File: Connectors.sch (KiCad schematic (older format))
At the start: 4 parts

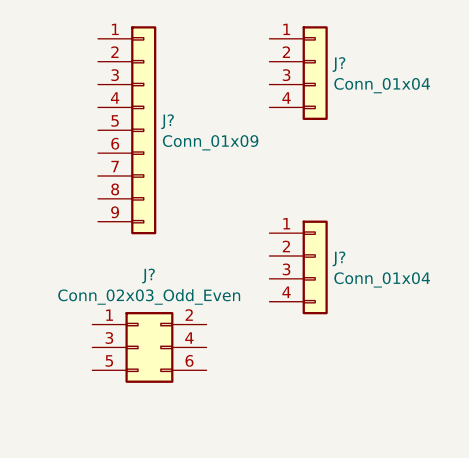
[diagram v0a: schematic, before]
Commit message: Arranged symbols
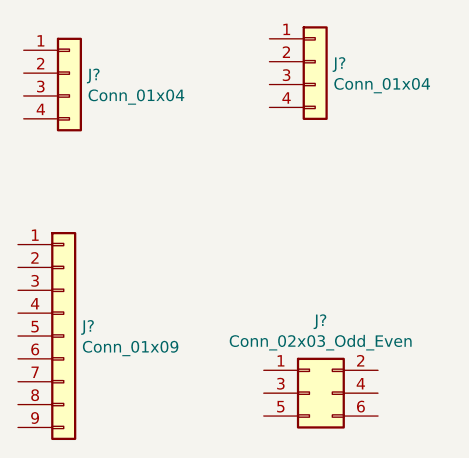
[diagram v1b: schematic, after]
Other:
- moved on the sheet: J?
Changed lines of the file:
@@
 L Connector_Generic:Conn_01x09 J?
 U 1 1 5CE3D253
-P 5175 2850
-F 0 "J?" H 5255 2892 50  0000 L CNN
-F 1 "Conn_01x09" H 5255 2801 50  0000 L CNN
-F 2 "" H 5175 2850 50  0001 C CNN
-F 3 "~" H 5175 2850 50  0001 C CNN
-	1    5175 2850
+P 4825 3750
+F 0 "J?" H 4905 3792 50  0000 L CNN
+F 1 "Conn_01x09" H 4905 3701 50  0000 L CNN
+F 2 "" H 4825 3750 50  0001 C CNN
+F 3 "~" H 4825 3750 50  0001 C CNN
+	1    4825 3750
 	1    0    0    -1
 $EndComp
@@
 L Connector_Generic:Conn_02x03_Odd_Even J?
 U 1 1 5CE3EBBD
-P 5150 3800
-F 0 "J?" H 5200 4117 50  0000 C CNN
-F 1 "Conn_02x03_Odd_Even" H 5200 4026 50  0000 C CNN
-F 2 "" H 5150 3800 50  0001 C CNN
-F 3 "~" H 5150 3800 50  0001 C CNN
-	1    5150 3800
+P 5900 4000
+F 0 "J?" H 5950 4317 50  0000 C CNN
+F 1 "Conn_02x03_Odd_Even" H 5950 4226 50  0000 C CNN
+F 2 "" H 5900 4000 50  0001 C CNN
+F 3 "~" H 5900 4000 50  0001 C CNN
+	1    5900 4000
 	1    0    0    -1
 $EndComp
@@
 L Connector_Generic:Conn_01x04 J?
 U 1 1 5CE40335
-P 5925 3400
-F 0 "J?" H 6005 3392 50  0000 L CNN
-F 1 "Conn_01x04" H 6005 3301 50  0000 L CNN
-F 2 "" H 5925 3400 50  0001 C CNN
-F 3 "~" H 5925 3400 50  0001 C CNN
-	1    5925 3400
+P 4850 2600
+F 0 "J?" H 4930 2592 50  0000 L CNN
+F 1 "Conn_01x04" H 4930 2501 50  0000 L CNN
+F 2 "" H 4850 2600 50  0001 C CNN
+F 3 "~" H 4850 2600 50  0001 C CNN
+	1    4850 2600
 	1    0    0    -1
 $EndComp
